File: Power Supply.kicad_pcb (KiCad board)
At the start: 2 copper layers, 160 x 100 mm, 4 parts

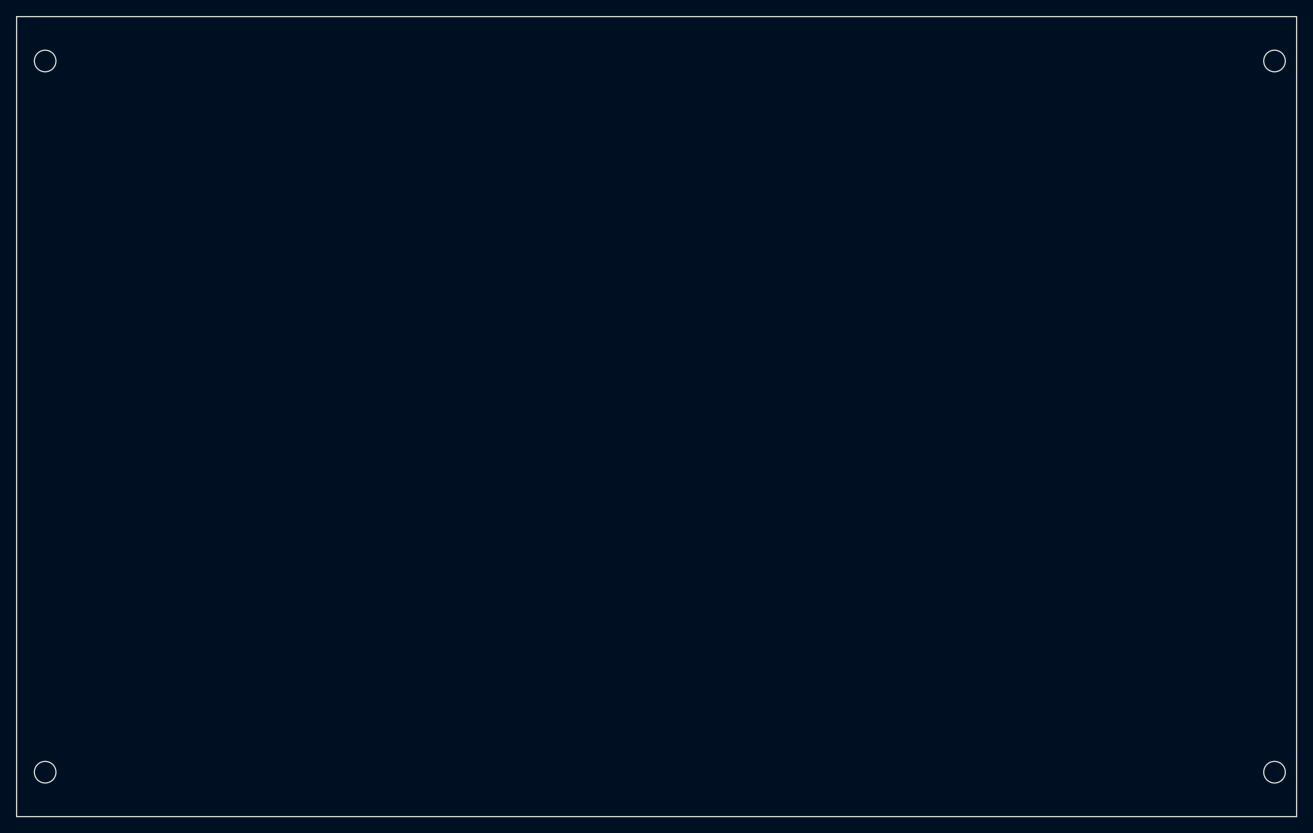
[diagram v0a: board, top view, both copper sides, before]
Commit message: Power Supplie Board V1.00
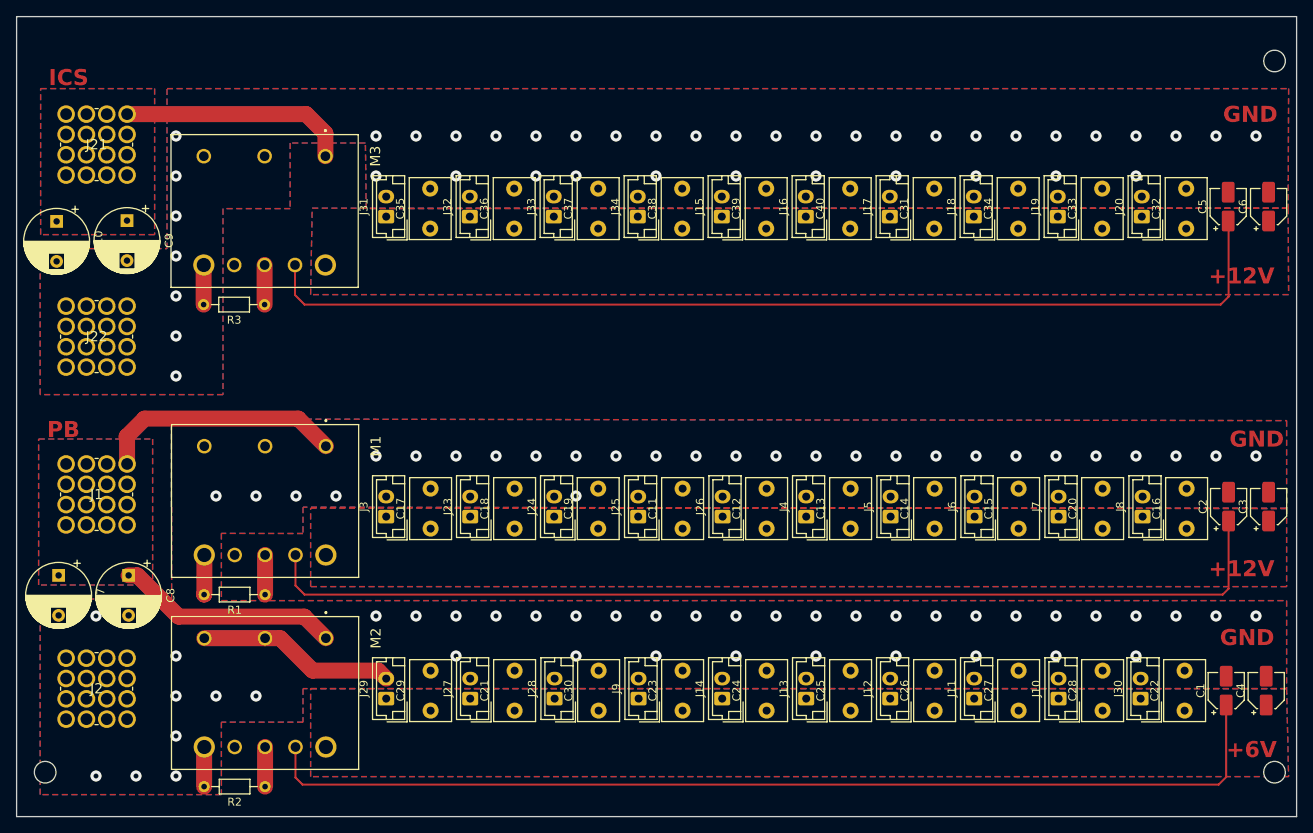
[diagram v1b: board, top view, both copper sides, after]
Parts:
- removed MH1: MountingHole_2.7mm_M2.5_DIN965, MountingHole:MountingHole_2.7mm_M2.5_DIN965
- added C1: 100nF, Capacitor_SMD:CP_Elec_4x5.8, F.Cu at (206.2, 129.2)
- added C10: 100uF, Capacitor_THT:CP_Radial_D8.0mm_P5.00mm, F.Cu at (60.0, 70.6)
- added C11: 1nF, Capacitor_THT:C_Disc_D7.5mm_W5.0mm_P5.00mm, F.Cu at (138.2, 109.0)
- added C12: 1nF, Capacitor_THT:C_Disc_D7.5mm_W5.0mm_P5.00mm, F.Cu at (148.8, 109.0)
- added C13: 1nF, Capacitor_THT:C_Disc_D7.5mm_W5.0mm_P5.00mm, F.Cu at (159.2, 109.0)
- added C14: 1nF, Capacitor_THT:C_Disc_D7.5mm_W5.0mm_P5.00mm, F.Cu at (169.8, 109.0)
- added C15: 1nF, Capacitor_THT:C_Disc_D7.5mm_W5.0mm_P5.00mm, F.Cu at (180.2, 109.0)
- added C16: 1nF, Capacitor_THT:C_Disc_D7.5mm_W5.0mm_P5.00mm, F.Cu at (201.2, 109.0)
- added C17: 1nF, Capacitor_THT:C_Disc_D7.5mm_W5.0mm_P5.00mm, F.Cu at (106.8, 109.0)
- added C18: 1nF, Capacitor_THT:C_Disc_D7.5mm_W5.0mm_P5.00mm, F.Cu at (117.2, 109.0)
- added C19: 1nF, Capacitor_THT:C_Disc_D7.5mm_W5.0mm_P5.00mm, F.Cu at (127.7, 109.0)
- added C2: 100nF, Capacitor_SMD:CP_Elec_4x5.8, F.Cu at (206.5, 106.2)
- added C20: 1nF, Capacitor_THT:C_Disc_D7.5mm_W5.0mm_P5.00mm, F.Cu at (190.8, 109.0)
- added C21: 1nF, Capacitor_THT:C_Disc_D7.5mm_W5.0mm_P5.00mm, F.Cu at (117.2, 131.8)
- added C22: 1nF, Capacitor_THT:C_Disc_D7.5mm_W5.0mm_P5.00mm, F.Cu at (201.0, 131.8)
- added C23: 1nF, Capacitor_THT:C_Disc_D7.5mm_W5.0mm_P5.00mm, F.Cu at (138.2, 131.8)
- added C24: 1nF, Capacitor_THT:C_Disc_D7.5mm_W5.0mm_P5.00mm, F.Cu at (148.8, 131.8)
- added C25: 1nF, Capacitor_THT:C_Disc_D7.5mm_W5.0mm_P5.00mm, F.Cu at (159.2, 131.8)
- added C26: 1nF, Capacitor_THT:C_Disc_D7.5mm_W5.0mm_P5.00mm, F.Cu at (169.8, 131.8)
- added C27: 1nF, Capacitor_THT:C_Disc_D7.5mm_W5.0mm_P5.00mm, F.Cu at (180.2, 131.8)
- added C28: 1nF, Capacitor_THT:C_Disc_D7.5mm_W5.0mm_P5.00mm, F.Cu at (190.8, 131.8)
- added C29: 1nF, Capacitor_THT:C_Disc_D7.5mm_W5.0mm_P5.00mm, F.Cu at (106.8, 131.8)
- added C3: 22uF, Capacitor_SMD:CP_Elec_4x5.7, F.Cu at (211.5, 106.2)
- added C30: 1nF, Capacitor_THT:C_Disc_D7.5mm_W5.0mm_P5.00mm, F.Cu at (127.8, 131.8)
- added C31: 1nF, Capacitor_THT:C_Disc_D7.5mm_W5.0mm_P5.00mm, F.Cu at (169.7, 71.5)
- added C32: 1nF, Capacitor_THT:C_Disc_D7.5mm_W5.0mm_P5.00mm, F.Cu at (201.2, 71.5)
- added C33: 1nF, Capacitor_THT:C_Disc_D7.5mm_W5.0mm_P5.00mm, F.Cu at (190.7, 71.5)
- added C34: 1nF, Capacitor_THT:C_Disc_D7.5mm_W5.0mm_P5.00mm, F.Cu at (180.2, 71.5)
- added C35: 1nF, Capacitor_THT:C_Disc_D7.5mm_W5.0mm_P5.00mm, F.Cu at (106.7, 71.5)
- added C36: 1nF, Capacitor_THT:C_Disc_D7.5mm_W5.0mm_P5.00mm, F.Cu at (117.2, 71.5)
- added C37: 1nF, Capacitor_THT:C_Disc_D7.5mm_W5.0mm_P5.00mm, F.Cu at (127.7, 71.5)
- added C38: 1nF, Capacitor_THT:C_Disc_D7.5mm_W5.0mm_P5.00mm, F.Cu at (138.2, 71.5)
- added C39: 1nF, Capacitor_THT:C_Disc_D7.5mm_W5.0mm_P5.00mm, F.Cu at (148.7, 71.5)
- added C4: 22uF, Capacitor_SMD:CP_Elec_4x5.7, F.Cu at (211.2, 129.2)
- added C40: 1nF, Capacitor_THT:C_Disc_D7.5mm_W5.0mm_P5.00mm, F.Cu at (159.2, 71.5)
- added C5: 100nF, Capacitor_SMD:CP_Elec_4x5.8, F.Cu at (206.4, 68.8)
- added C6: 22uF, Capacitor_SMD:CP_Elec_4x5.7, F.Cu at (211.5, 68.8)
- added C7: 100uF, Capacitor_THT:CP_Radial_D8.0mm_P5.00mm, F.Cu at (60.2, 114.8)
- added C8: 100uF, Capacitor_THT:CP_Radial_D8.0mm_P5.00mm, F.Cu at (69.0, 114.8)
- added C9: 100uF, Capacitor_THT:CP_Radial_D8.0mm_P5.00mm, F.Cu at (68.8, 70.5)
- added J1: ~, My Global Library:7461383, F.Cu at (61.2, 108.5)
- added J10: Connector, Connector_JST:JST_EH_B2B-EH-A_1x02_P2.50mm_Vertical, F.Cu at (185.2, 130.2)
- added J11: Connector, Connector_JST:JST_EH_B2B-EH-A_1x02_P2.50mm_Vertical, F.Cu at (174.7, 130.2)
- added J12: Connector, Connector_JST:JST_EH_B2B-EH-A_1x02_P2.50mm_Vertical, F.Cu at (164.2, 130.2)
- added J13: Connector, Connector_JST:JST_EH_B2B-EH-A_1x02_P2.50mm_Vertical, F.Cu at (153.7, 130.2)
- added J14: Connector, Connector_JST:JST_EH_B2B-EH-A_1x02_P2.50mm_Vertical, F.Cu at (143.2, 130.2)
- added J15: Connector, Connector_JST:JST_EH_B2B-EH-A_1x02_P2.50mm_Vertical, F.Cu at (143.2, 70.0)
- added J16: Connector, Connector_JST:JST_EH_B2B-EH-A_1x02_P2.50mm_Vertical, F.Cu at (153.7, 70.0)
- added J17: Connector, Connector_JST:JST_EH_B2B-EH-A_1x02_P2.50mm_Vertical, F.Cu at (164.2, 70.0)
- added J18: Connector, Connector_JST:JST_EH_B2B-EH-A_1x02_P2.50mm_Vertical, F.Cu at (174.7, 70.0)
- added J19: Connector, Connector_JST:JST_EH_B2B-EH-A_1x02_P2.50mm_Vertical, F.Cu at (185.2, 70.0)
- added J2: ~, My Global Library:7461383, F.Cu at (61.2, 132.8)
- added J20: Connector, Connector_JST:JST_EH_B2B-EH-A_1x02_P2.50mm_Vertical, F.Cu at (195.7, 70.0)
- added J21: ~, My Global Library:7461383, F.Cu at (61.2, 64.8)
- added J22: ~, My Global Library:7461383, F.Cu at (61.2, 88.8)
- added J23: Connector, Connector_JST:JST_EH_B2B-EH-A_1x02_P2.50mm_Vertical, F.Cu at (111.7, 107.5)
- added J24: Connector, Connector_JST:JST_EH_B2B-EH-A_1x02_P2.50mm_Vertical, F.Cu at (122.2, 107.5)
- added J25: Connector, Connector_JST:JST_EH_B2B-EH-A_1x02_P2.50mm_Vertical, F.Cu at (132.7, 107.5)
- added J26: Connector, Connector_JST:JST_EH_B2B-EH-A_1x02_P2.50mm_Vertical, F.Cu at (143.2, 107.5)
- added J27: Connector, Connector_JST:JST_EH_B2B-EH-A_1x02_P2.50mm_Vertical, F.Cu at (111.7, 130.2)
- added J28: Connector, Connector_JST:JST_EH_B2B-EH-A_1x02_P2.50mm_Vertical, F.Cu at (122.2, 130.2)
- added J29: Connector, Connector_JST:JST_EH_B2B-EH-A_1x02_P2.50mm_Vertical, F.Cu at (101.2, 130.2)
- added J3: Connector, Connector_JST:JST_EH_B2B-EH-A_1x02_P2.50mm_Vertical, F.Cu at (101.2, 107.5)
- added J30: Connector, Connector_JST:JST_EH_B2B-EH-A_1x02_P2.50mm_Vertical, F.Cu at (195.5, 130.2)
- added J31: Connector, Connector_JST:JST_EH_B2B-EH-A_1x02_P2.50mm_Vertical, F.Cu at (101.2, 70.0)
- added J32: Connector, Connector_JST:JST_EH_B2B-EH-A_1x02_P2.50mm_Vertical, F.Cu at (111.7, 70.0)
- added J33: Connector, Connector_JST:JST_EH_B2B-EH-A_1x02_P2.50mm_Vertical, F.Cu at (122.2, 70.0)
- added J34: Connector, Connector_JST:JST_EH_B2B-EH-A_1x02_P2.50mm_Vertical, F.Cu at (132.7, 70.0)
- added J4: Connector, Connector_JST:JST_EH_B2B-EH-A_1x02_P2.50mm_Vertical, F.Cu at (153.7, 107.5)
- added J5: Connector, Connector_JST:JST_EH_B2B-EH-A_1x02_P2.50mm_Vertical, F.Cu at (164.2, 107.5)
- added J6: Connector, Connector_JST:JST_EH_B2B-EH-A_1x02_P2.50mm_Vertical, F.Cu at (174.8, 107.5)
- added J7: Connector, Connector_JST:JST_EH_B2B-EH-A_1x02_P2.50mm_Vertical, F.Cu at (185.2, 107.5)
- added J8: Connector, Connector_JST:JST_EH_B2B-EH-A_1x02_P2.50mm_Vertical, F.Cu at (195.8, 107.5)
- added J9: Connector, Connector_JST:JST_EH_B2B-EH-A_1x02_P2.50mm_Vertical, F.Cu at (132.8, 130.2)
- added M1: TDK, My Global Library:I3A4W005A150V001R, F.Cu at (93.7, 98.7)
- added M2: TDK, My Global Library:I3A4W005A150V001R, F.Cu at (93.7, 122.7)
- added M3: TDK, My Global Library:I3A4W005A150V001R, F.Cu at (93.6, 62.5)
- added R1: 1.82k, Resistor_THT:R_Axial_DIN0204_L3.6mm_D1.6mm_P7.62mm_Horizontal, F.Cu at (86.1, 117.2)
- added R2: 5.9k, Resistor_THT:R_Axial_DIN0204_L3.6mm_D1.6mm_P7.62mm_Horizontal, F.Cu at (86.1, 141.2)
- added R3: 1.82k, Resistor_THT:R_Axial_DIN0204_L3.6mm_D1.6mm_P7.62mm_Horizontal, F.Cu at (86.0, 81.0)
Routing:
- net Vdrive: track 0.00 -> 130.8 mm
- net +6V: track 0.00 -> 129.9 mm
- net +12V: track 0.00 -> 129.7 mm
- net Net-(J1-0): track 0.00 -> 58.6 mm
- net GND1: track 0.00 -> 34.7 mm, vias 0 -> 69
- net Net-(J21-0): track 0.00 -> 28.6 mm
- net GND2: track 0.00 -> 4.96 mm, vias 0 -> 41
- net Net-(M3-TRIM): track 0.00 -> 4.95 mm
- net Net-(M1-TRIM): track 0.00 -> 4.95 mm
- net Net-(M2-TRIM): track 0.00 -> 4.95 mm
- added copper zone on B.Cu, net +12V
- added copper zone on F.Cu, net +12V
- added copper zone on B.Cu, net +6V
- added copper zone on F.Cu, net +6V
- added copper zone on B.Cu, net GND1
- added copper zone on F.Cu, net GND1
- added copper zone on B.Cu, net GND2
- added copper zone on F.Cu, net GND2
- added copper zone on B.Cu, net Net-(J1-0)
- added copper zone on F.Cu, net Net-(J1-0)
- added copper zone on B.Cu, net Net-(J21-0)
- added copper zone on F.Cu, net Net-(J21-0)
- added copper zone on B.Cu, net Vdrive
- added copper zone on F.Cu, net Vdrive
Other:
- board text added: "+12V"
- board text added: "+6V"
- board text added: "GND"
- board text added: "ICS"
- board text added: "PB"
